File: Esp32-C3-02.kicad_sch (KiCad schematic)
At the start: 0 parts

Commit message: Schematic update
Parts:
- added J3: GSD09002SEU, GSD09002SEU:AMPHENOL_GSD09002SEU, symbol GSD09002SEU:GSD09002SEU
- added U2: USBLC6-2SC6, Package_TO_SOT_SMD:SOT-23-6, symbol Power_Protection:USBLC6-2SC6
- added U3: ESP32-C3-WROOM-02, RF_Module:ESP32-C3-WROOM-02, symbol RF_Module:ESP32-C3-WROOM-02
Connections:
- new net: U3.19 (GND), U3.9 (GND)

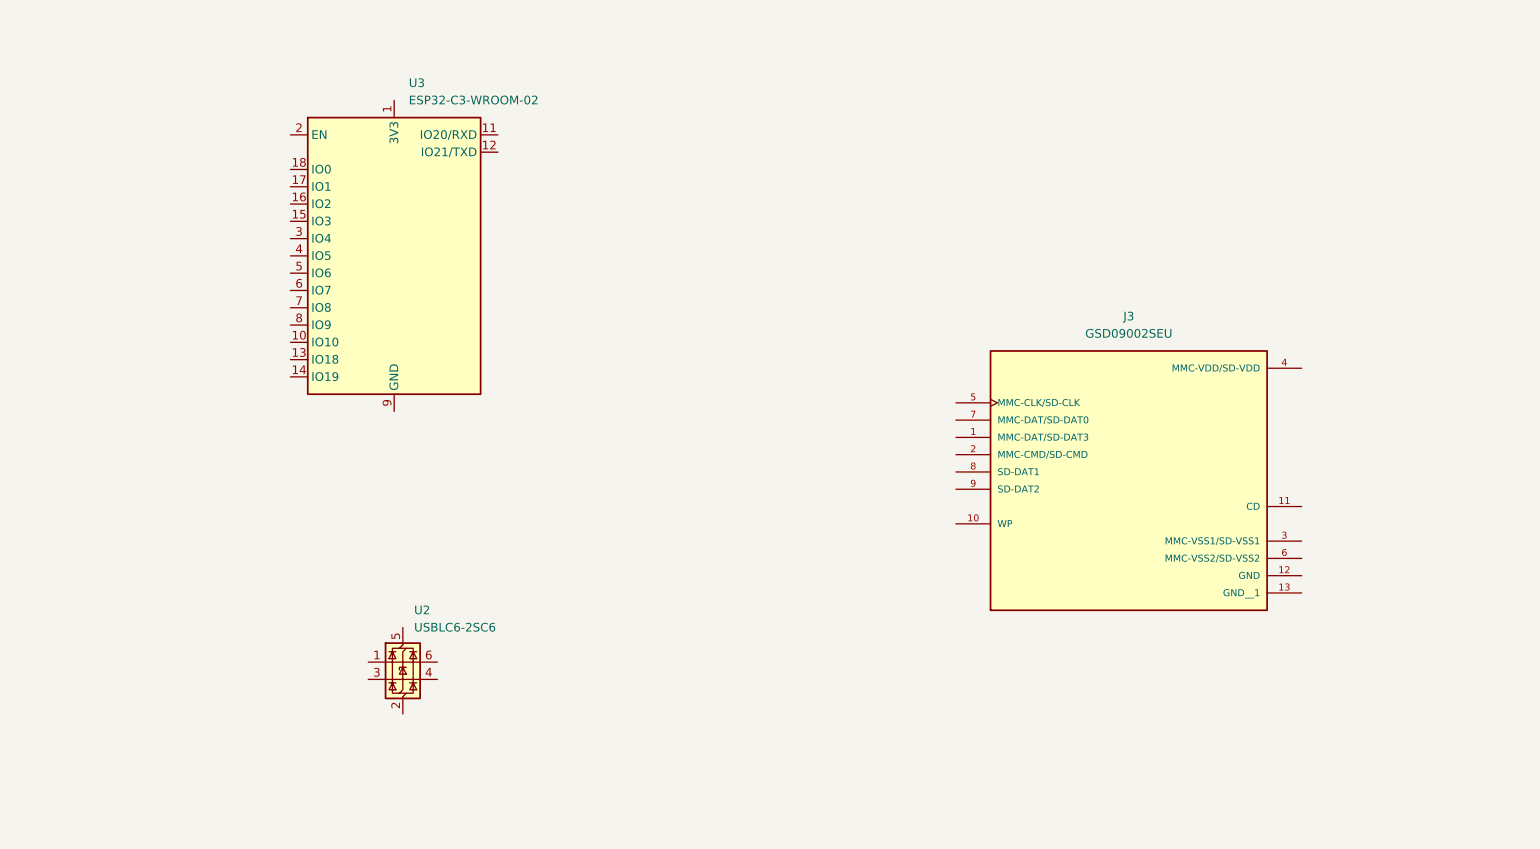
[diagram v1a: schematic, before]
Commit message: esp32 circuitry design
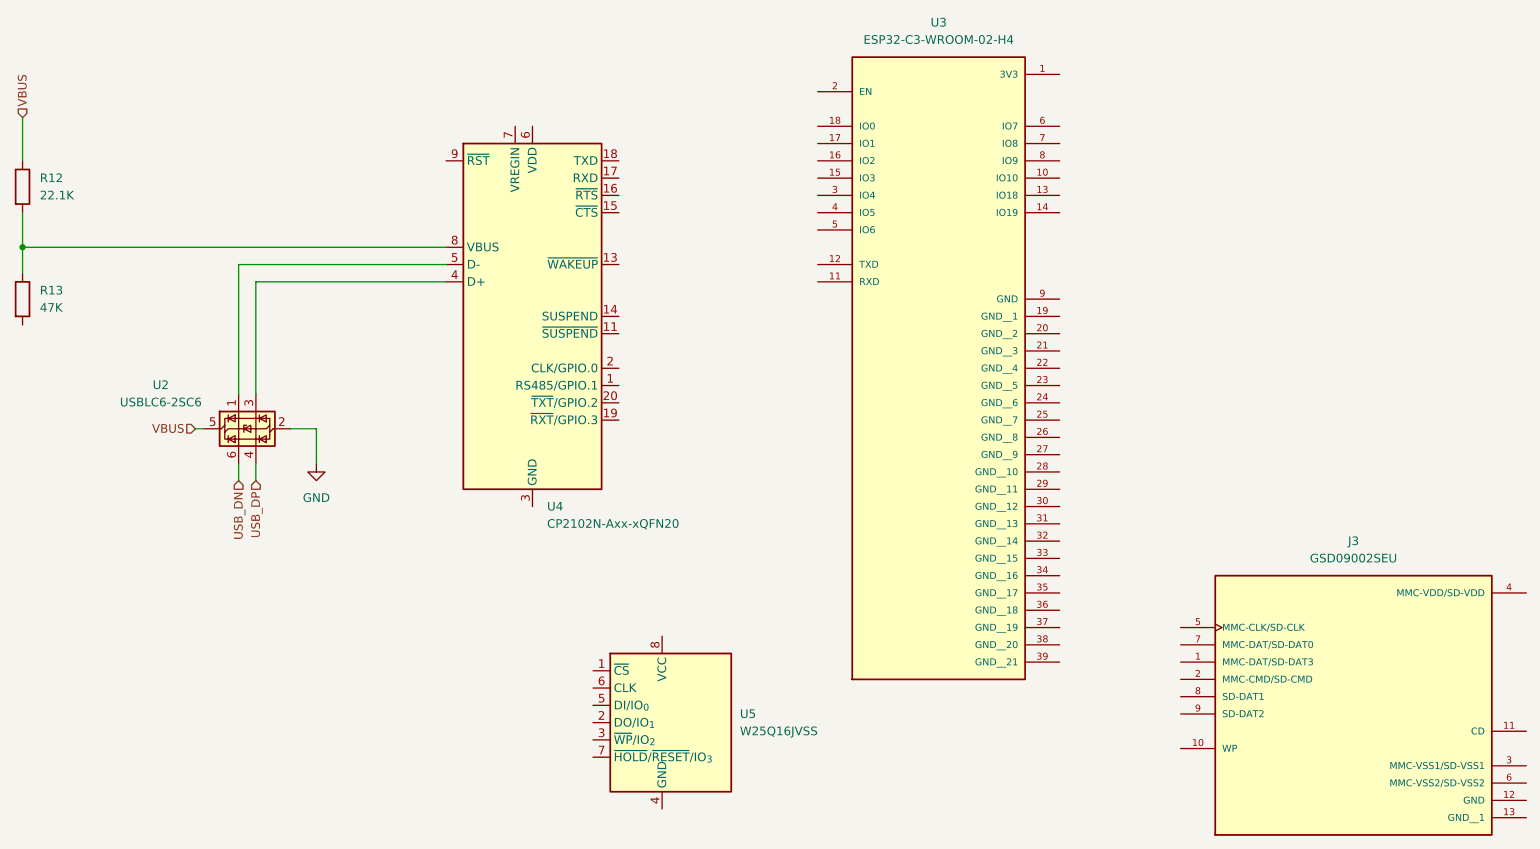
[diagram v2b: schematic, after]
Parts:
- removed U3: ESP32-C3-WROOM-02, RF_Module:ESP32-C3-WROOM-02, symbol RF_Module:ESP32-C3-WROOM-02
- added R12: 22.1K, symbol Device:R
- added R13: 47K, symbol Device:R
- added U3: ESP32-C3-WROOM-02-H4, ESP32-C3-WROOM-02-H4:MODULE_ESP32-C3-WROOM-02-H4, symbol ESP32-C3-WROOM-02-H4:ESP32-C3-WROOM-02-H4
- added U4: CP2102N-Axx-xQFN20, Package_DFN_QFN:SiliconLabs_QFN-20-1EP_3x3mm_P0.5mm, symbol Interface_USB:CP2102N-Axx-xQFN20
- added U5: W25Q16JVSS, Package_SO:SOIC-8_5.3x5.3mm_P1.27mm, symbol Memory_Flash:W25Q16JVSS
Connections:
- net at U2.1 (I/O1): now also U4.5 (D-)
- net GND: now reaches U2.2 (GND)
- net at U2.3 (I/O2): now also U4.4 (D+)
- net USB_DP: now reaches U2.4 (I/O2)
- net VBUS: now reaches U2.5 (VBUS)
- net VBUS: now also R12.1
- net USB_DN: now reaches U2.6 (I/O1)
- new net: U4.12 (GND), U4.21 (GND), U4.3 (GND)
- new net: R12.2, R13.1, U4.8 (VBUS)
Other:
- moved on the sheet: J3, U2
